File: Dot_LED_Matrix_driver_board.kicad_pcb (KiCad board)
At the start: 2 copper layers, 60.2 x 60.2 mm, 9 parts, among them U1 MAX7219

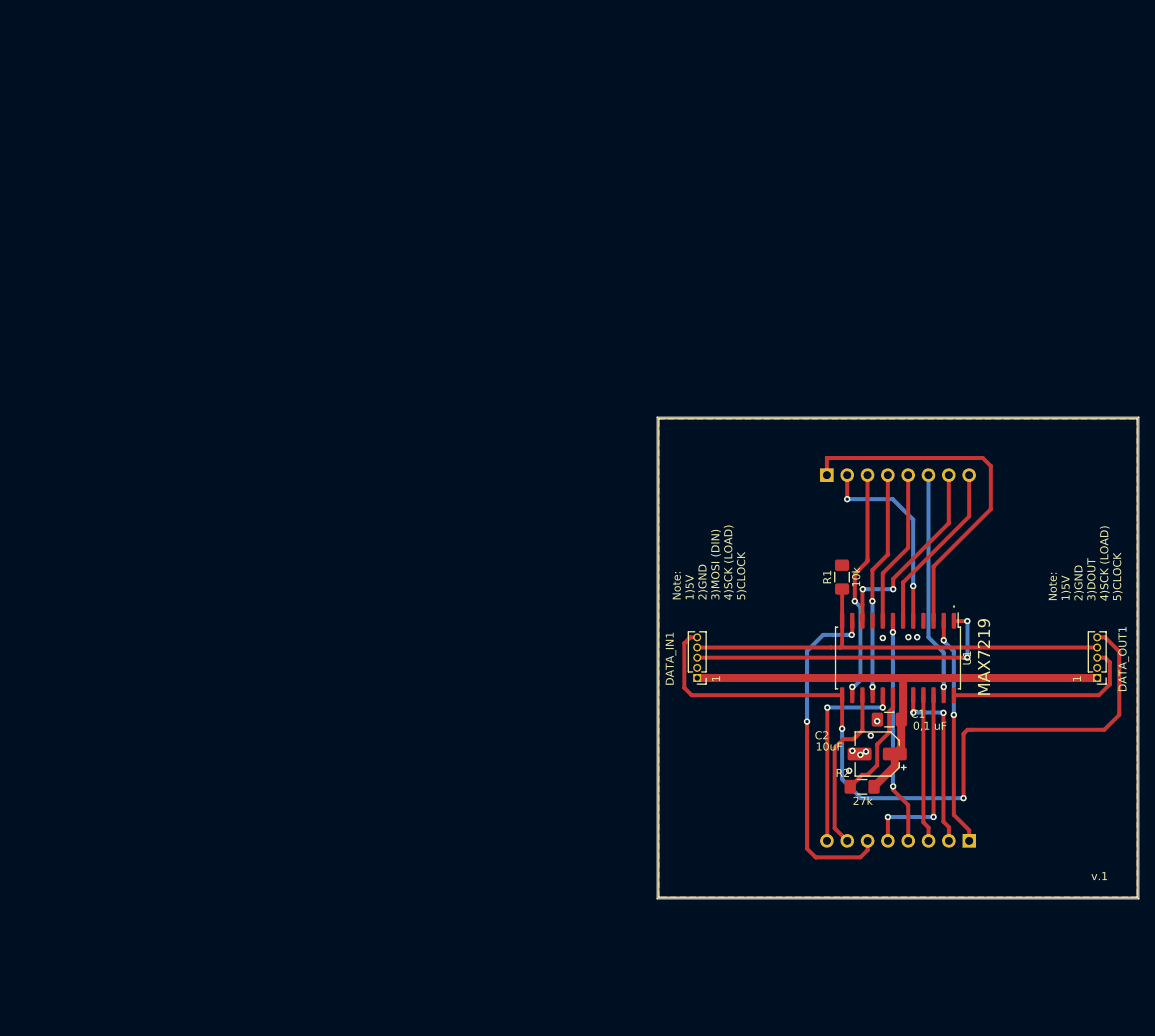
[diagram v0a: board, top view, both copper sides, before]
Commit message: Signed-off-by: Martynas Sprogys <martynas2580@gmail.com>
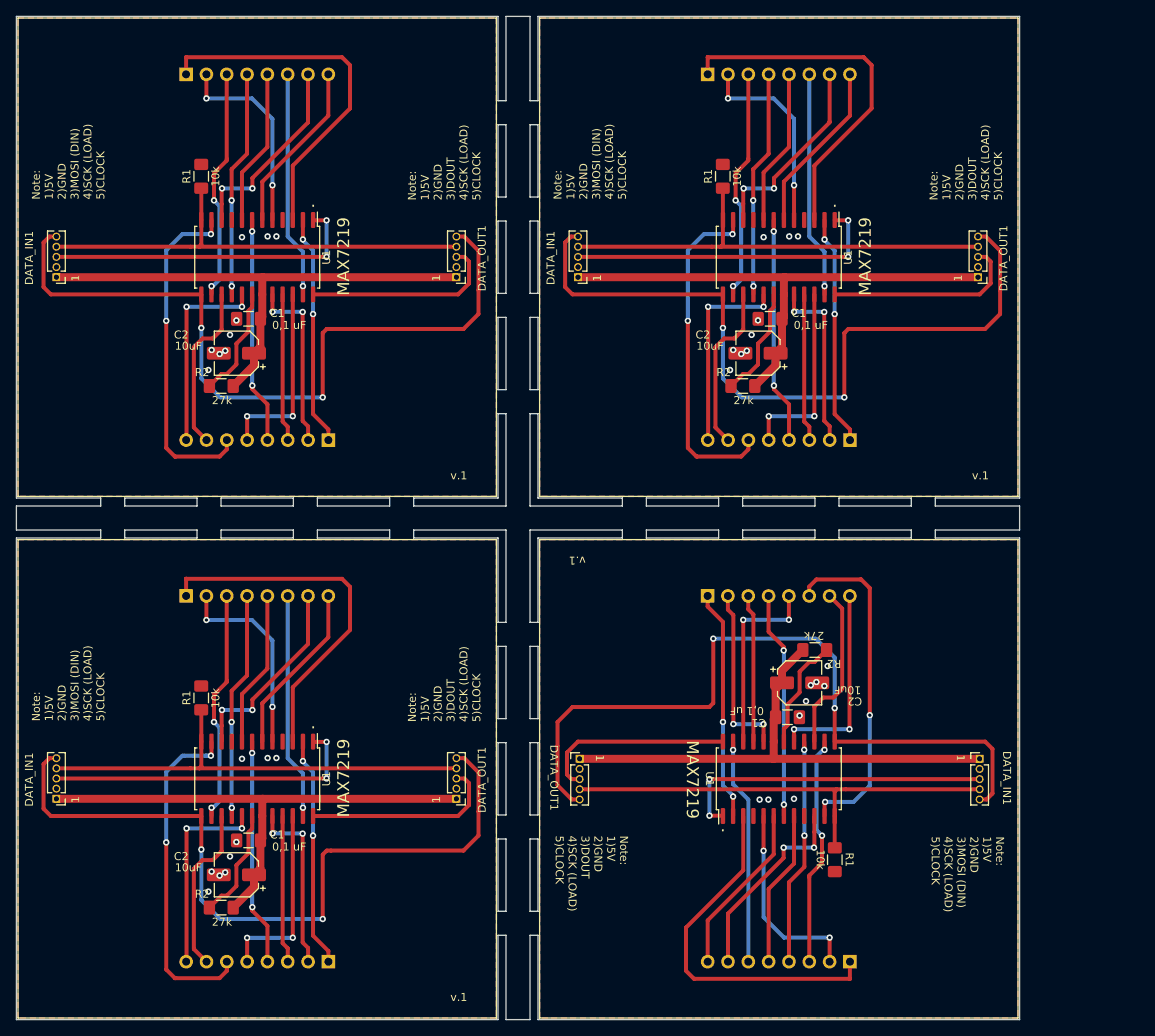
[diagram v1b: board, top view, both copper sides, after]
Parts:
- removed the Anodes(+)1 at (121.2, 77.2)
- removed the C1 at (129.0, 107.8)
- removed the C2 at (127.5, 112.1)
- removed the Cathodes(-)1 at (139.0, 123.0)
- removed the DATA_IN1 at (105.0, 102.6)
- removed the DATA_OUT1 at (155.0, 102.6)
- removed the R1 at (123.1, 90.0)
- removed the R2 at (125.6, 116.2)
- removed the U1 at (130.1, 100.1)
- added Anodes(+)1: pin header 2.54 mm, Connector_PinHeader_2.54mm:PinHeader_1x08_P2.54mm_Vertical, B.Cu at (41.1, 92.3)
- added Anodes(+)1: pin header 2.54 mm, Connector_PinHeader_2.54mm:PinHeader_1x08_P2.54mm_Vertical, B.Cu at (41.1, 27.1)
- added Anodes(+)1: pin header 2.54 mm, Connector_PinHeader_2.54mm:PinHeader_1x08_P2.54mm_Vertical, B.Cu at (106.3, 27.1)
- added Anodes(+)1: pin header 2.54 mm, Connector_PinHeader_2.54mm:PinHeader_1x08_P2.54mm_Vertical, B.Cu at (124.1, 138.1)
- added C1: 0,1uF, Capacitor_SMD:C_1206_3216Metric_Pad1.42x1.75mm_HandSolder, F.Cu at (116.3, 107.5)
- added C1: 0,1uF, Capacitor_SMD:C_1206_3216Metric_Pad1.42x1.75mm_HandSolder, F.Cu at (48.9, 57.7)
- added C1: 0,1uF, Capacitor_SMD:C_1206_3216Metric_Pad1.42x1.75mm_HandSolder, F.Cu at (114.1, 57.7)
- added C1: 0,1uF, Capacitor_SMD:C_1206_3216Metric_Pad1.42x1.75mm_HandSolder, F.Cu at (48.9, 122.9)
- added C2: 10uF, Capacitor_SMD:CP_Elec_5x3, F.Cu at (47.4, 62.0)
- added C2: 10uF, Capacitor_SMD:CP_Elec_5x3, F.Cu at (117.8, 103.2)
- added C2: 10uF, Capacitor_SMD:CP_Elec_5x3, F.Cu at (47.4, 127.2)
- added C2: 10uF, Capacitor_SMD:CP_Elec_5x3, F.Cu at (112.6, 62.0)
- added Cathodes(-)1: pin header 2.54 mm, Connector_PinHeader_2.54mm:PinHeader_1x08_P2.54mm_Vertical, B.Cu at (58.9, 72.9)
- added Cathodes(-)1: pin header 2.54 mm, Connector_PinHeader_2.54mm:PinHeader_1x08_P2.54mm_Vertical, B.Cu at (58.9, 138.1)
- added Cathodes(-)1: pin header 2.54 mm, Connector_PinHeader_2.54mm:PinHeader_1x08_P2.54mm_Vertical, B.Cu at (106.3, 92.3)
- added Cathodes(-)1: pin header 2.54 mm, Connector_PinHeader_2.54mm:PinHeader_1x08_P2.54mm_Vertical, B.Cu at (124.1, 72.9)
- added DATA_IN1: Conn_01x05, Connector_PinHeader_1.27mm:PinHeader_1x05_P1.27mm_Vertical, F.Cu at (24.9, 117.7)
- added DATA_IN1: Conn_01x05, Connector_PinHeader_1.27mm:PinHeader_1x05_P1.27mm_Vertical, F.Cu at (24.9, 52.5)
- added DATA_IN1: Conn_01x05, Connector_PinHeader_1.27mm:PinHeader_1x05_P1.27mm_Vertical, F.Cu at (90.1, 52.5)
- added DATA_IN1: Conn_01x05, Connector_PinHeader_1.27mm:PinHeader_1x05_P1.27mm_Vertical, F.Cu at (140.3, 112.7)
- added DATA_OUT1: Conn_01x05, Connector_PinHeader_1.27mm:PinHeader_1x05_P1.27mm_Vertical, F.Cu at (90.3, 112.7)
- added DATA_OUT1: Conn_01x05, Connector_PinHeader_1.27mm:PinHeader_1x05_P1.27mm_Vertical, F.Cu at (140.1, 52.5)
- added DATA_OUT1: Conn_01x05, Connector_PinHeader_1.27mm:PinHeader_1x05_P1.27mm_Vertical, F.Cu at (74.9, 117.7)
- added DATA_OUT1: Conn_01x05, Connector_PinHeader_1.27mm:PinHeader_1x05_P1.27mm_Vertical, F.Cu at (74.9, 52.5)
- added R1: 10k, Resistor_SMD:R_1206_3216Metric_Pad1.42x1.75mm_HandSolder, F.Cu at (108.2, 39.9)
- added R1: 10k, Resistor_SMD:R_1206_3216Metric_Pad1.42x1.75mm_HandSolder, F.Cu at (122.2, 125.3)
- added R1: 10k, Resistor_SMD:R_1206_3216Metric_Pad1.42x1.75mm_HandSolder, F.Cu at (43.0, 39.9)
- added R1: 10k, Resistor_SMD:R_1206_3216Metric_Pad1.42x1.75mm_HandSolder, F.Cu at (43.0, 105.1)
- added R2: 27k, Resistor_SMD:R_1206_3216Metric_Pad1.42x1.75mm_HandSolder, F.Cu at (45.5, 66.1)
- added R2: 27k, Resistor_SMD:R_1206_3216Metric_Pad1.42x1.75mm_HandSolder, F.Cu at (45.5, 131.3)
- added R2: 27k, Resistor_SMD:R_1206_3216Metric_Pad1.42x1.75mm_HandSolder, F.Cu at (110.7, 66.1)
- added R2: 27k, Resistor_SMD:R_1206_3216Metric_Pad1.42x1.75mm_HandSolder, F.Cu at (119.7, 99.1)
- added U1: MAX7219, Package_SO:SOP-24_7.5x15.4mm_P1.27mm, F.Cu at (50.0, 115.2)
- added U1: MAX7219, Package_SO:SOP-24_7.5x15.4mm_P1.27mm, F.Cu at (50.0, 50.0)
- added U1: MAX7219, Package_SO:SOP-24_7.5x15.4mm_P1.27mm, F.Cu at (115.2, 50.0)
- added U1: MAX7219, Package_SO:SOP-24_7.5x15.4mm_P1.27mm, F.Cu at (115.2, 115.2)
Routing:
- net Board_1-CK: track 0.00 -> 94.2 mm, vias 0 -> 2
- net Board_2-CK: track 0.00 -> 94.2 mm, vias 0 -> 2
- net Board_0-CK: track 0.00 -> 94.2 mm, vias 0 -> 2
- net CK: track 94.2 -> 0.00 mm, vias 2 -> 0
- net Board_3-CK: track 0.00 -> 94.2 mm, vias 0 -> 2
- net 5V: track 65.1 -> 0.00 mm
- net Board_3-5V: track 0.00 -> 65.1 mm
- net Board_2-5V: track 0.00 -> 65.1 mm
- net Board_1-5V: track 0.00 -> 65.1 mm
- net Board_0-5V: track 0.00 -> 65.1 mm
- net CS: track 57.4 -> 0.00 mm
- net Board_3-CS: track 0.00 -> 57.4 mm
- net Board_2-CS: track 0.00 -> 57.4 mm
- net Board_0-CS: track 0.00 -> 57.4 mm
- net Board_1-CS: track 0.00 -> 57.4 mm
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- added copper zone on B.Cu, net Board_0-GND
- added copper zone on F.Cu, net Board_0-GND
- added copper zone on B.Cu, net Board_1-GND
- added copper zone on F.Cu, net Board_1-GND
- added copper zone on B.Cu, net Board_2-GND
- added copper zone on F.Cu, net Board_2-GND
- added copper zone on B.Cu, net Board_3-GND
- added copper zone on F.Cu, net Board_3-GND
- removed copper zone on B.Cu, net GND
- removed copper zone on F.Cu, net GND
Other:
- board size 60.2 x 60.2 mm -> 125.4 x 125.4 mm
